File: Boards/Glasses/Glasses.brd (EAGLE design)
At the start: 157.5 x 68.6 mm, 260 parts, among them U1 APA1022020, U10 APA1022020, U100 APA1022020, U101 APA1022020, U102 APA1022020, U103 APA1022020, U104 APA1022020, U105 APA1022020, U106 APA1022020, U107 APA1022020, U108 APA1022020, U109 APA1022020, U11 APA1022020, U110 APA1022020, U111 APA1022020, U112 APA1022020, U113 APA1022020, U114 APA1022020, U115 APA1022020, U116 APA1022020, U117 APA1022020, U118 APA1022020, U119 APA1022020, U12 APA1022020, U120 APA1022020, U121 APA1022020, U122 APA1022020, U123 APA1022020, U124 APA1022020, U125 APA1022020, U126 APA1022020, U127 APA1022020, U128 APA1022020, U129 APA1022020, U13 APA1022020, U130 APA1022020, U131 APA1022020, U132 APA1022020, U133 APA1022020, U134 APA1022020, U135 APA1022020, U136 APA1022020, U137 APA1022020, U138 APA1022020, U139 APA1022020, U14 APA1022020, U140 APA1022020, U141 APA1022020, U142 APA1022020, U143 APA1022020, U144 APA1022020, U145 APA1022020, U146 APA1022020, U147 APA1022020, U148 APA1022020, U149 APA1022020, U15 APA1022020, U150 APA1022020, U151 APA1022020, U152 APA1022020, U153 APA1022020, U154 APA1022020, U155 APA1022020, U156 APA1022020, U157 APA1022020, U158 APA1022020, U159 APA1022020, U16 APA1022020, U160 APA1022020, U161 APA1022020, U162 APA1022020, U163 APA1022020, U164 APA1022020, U165 APA1022020, U166 APA1022020, U167 APA1022020, U168 APA1022020, U169 APA1022020, U17 APA1022020, U170 APA1022020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

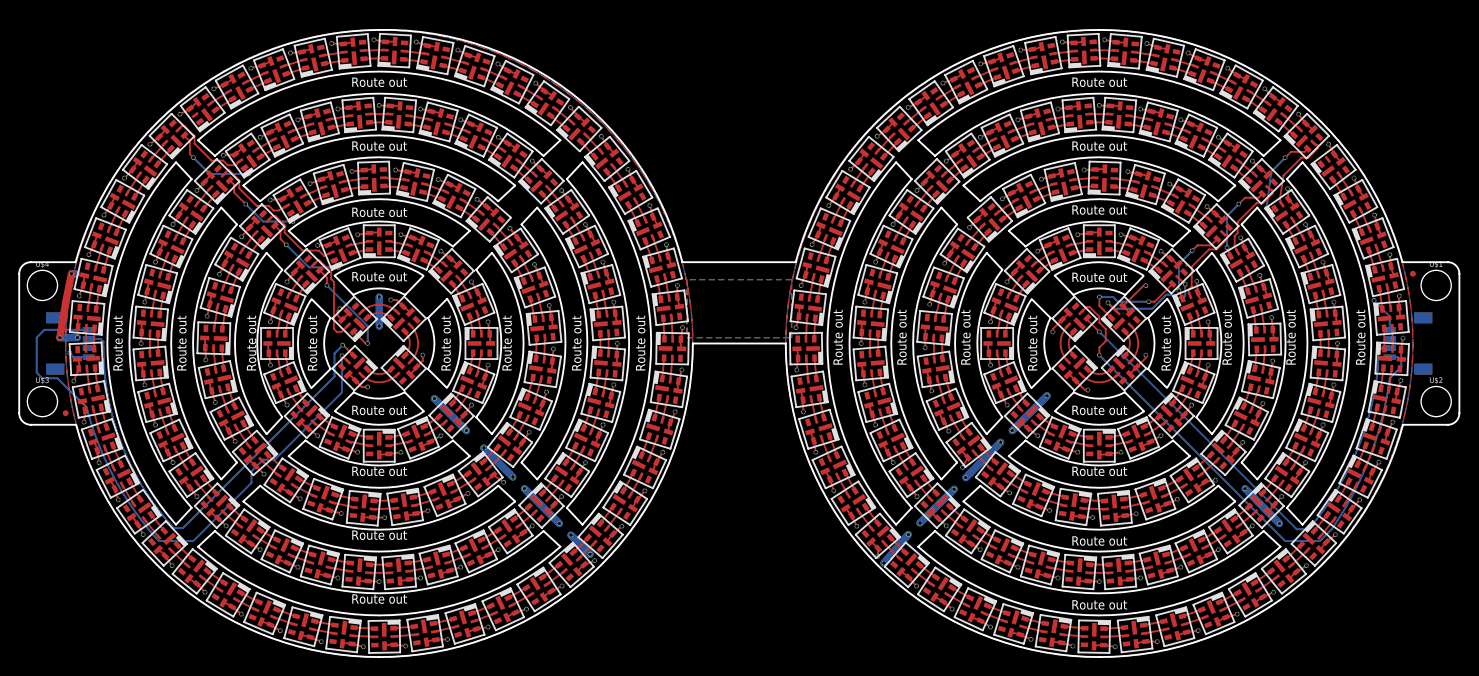
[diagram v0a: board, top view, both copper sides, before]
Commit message: adding gcode
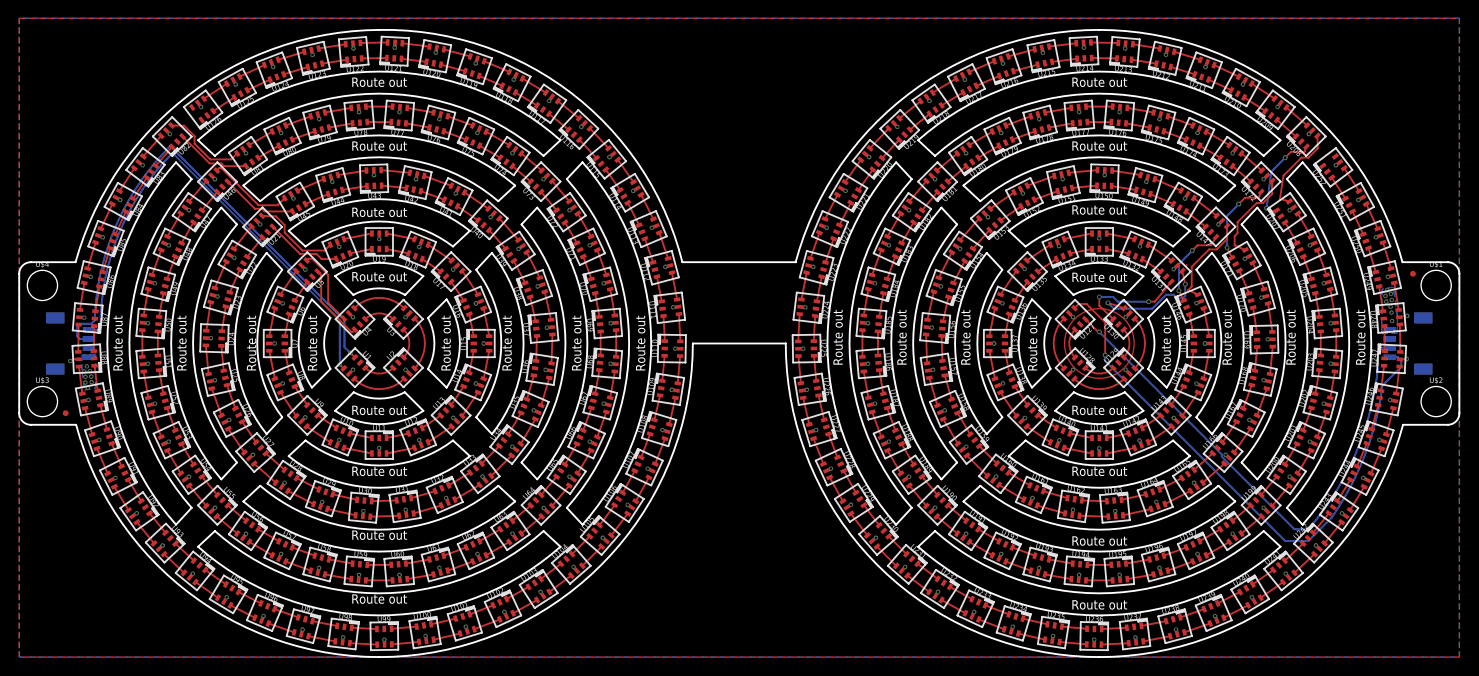
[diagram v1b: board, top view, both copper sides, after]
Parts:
- U1, U10, U100, U101, U102, U103, U104, U105, U106, U107, U108, U109, U11, U110, U111, U112, U113, U114, U115, U116, U117, U118, U119, U12, U120, U121, U122, U123, U124, U125, U126, U127, U128, U129, U13, U130, U131, U132, U133, U134, U135, U136, U137, U138, U139, U14, U140, U141, U142, U143, U144, U145, U146, U147, U148, U149, U15, U150, U151, U152, U153, U154, U155, U156, U157, U158, U159, U16, U160, U161, U162, U163, U164, U165, U166, U167, U168, U169, U17, U170, U171, U172, U173, U174, U175, U176, U177, U178, U179, U18, U180, U181, U182, U183, U184, U185, U186, U187, U188, U189, U19, U190, U191, U192, U193, U194, U195, U196, U197, U198, U199, U2, U20, U200, U201, U202, U203, U204, U205, U206, U207, U208, U209, U21, U210, U211, U212, U213, U214, U215, U216, U217, U218, U219, U22, U220, U221, U222, U223, U224, U225, U226, U227, U228, U229, U23, U230, U231, U232, U233, U234, U235, U236, U237, U238, U239, U24, U240, U241, U242, U243, U244, U245, U246, U247, U248, U249, U25, U250, U251, U252, U26, U27, U28, U29, U3, U30, U31, U32, U33, U34, U35, U36, U37, U38, U39, U4, U40, U41, U42, U43, U44, U45, U46, U47, U48, U49, U5, U50, U51, U52, U53, U54, U55, U56, U57, U58, U59, U6, U60, U61, U62, U63, U64, U65, U66, U67, U68, U69, U7, U70, U71, U72, U73, U74, U75, U76, U77, U78, U79, U8, U80, U81, U82, U83, U84, U85, U86, U87, U88, U89, U9, U90, U91, U92, U93, U94, U95, U96, U97, U98, U99: value APA1022020 -> APA102-2020; device 1_BES_Optoelectronics:APA102-2020 -> SparkFun-LED:APA102-2020
- turned U1 to 315 degrees
- turned U10 to 337.5 degrees
- turned U100 to 9 degrees
- turned U101 to 17 degrees
- turned U102 to 25 degrees
- turned U103 to 33 degrees
- turned U104 to 41 degrees
- turned U105 to 49 degrees
- turned U106 to 57 degrees
- turned U107 to 65 degrees
- turned U108 to 73 degrees
- turned U109 to 81 degrees
- turned U11 to 0 degrees
- turned U110 to 89 degrees
- turned U111 to 97 degrees
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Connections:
- net GND: no longer U1.GNDPAD, U10.GNDPAD, U100.GNDPAD, U101.GNDPAD, U102.GNDPAD, U103.GNDPAD, U104.GNDPAD, U105.GNDPAD, U106.GNDPAD, U107.GNDPAD, U108.GNDPAD, U109.GNDPAD, U11.GNDPAD, U110.GNDPAD, U111.GNDPAD, U112.GNDPAD, U113.GNDPAD, U114.GNDPAD, U115.GNDPAD, U116.GNDPAD, U117.GNDPAD, U118.GNDPAD, U119.GNDPAD, U12.GNDPAD, U120.GNDPAD, U121.GNDPAD, U122.GNDPAD, U123.GNDPAD, U124.GNDPAD, U125.GNDPAD, U126.GNDPAD, U127.GNDPAD, U128.GNDPAD, U129.GNDPAD, U13.GNDPAD, U130.GNDPAD, U131.GNDPAD, U132.GNDPAD, U133.GNDPAD, U134.GNDPAD, U135.GNDPAD, U136.GNDPAD, U137.GNDPAD, U138.GNDPAD, U139.GNDPAD, U14.GNDPAD, U140.GNDPAD, U141.GNDPAD, U142.GNDPAD, U143.GNDPAD, U144.GNDPAD, U145.GNDPAD, U146.GNDPAD, U147.GNDPAD, U148.GNDPAD, U149.GNDPAD, U15.GNDPAD, U150.GNDPAD, U151.GNDPAD, U152.GNDPAD, U153.GNDPAD, U154.GNDPAD, U155.GNDPAD, U156.GNDPAD, U157.GNDPAD, U158.GNDPAD, U159.GNDPAD, U16.GNDPAD, U160.GNDPAD, U161.GNDPAD, U162.GNDPAD, U163.GNDPAD, U164.GNDPAD, U165.GNDPAD, U166.GNDPAD, U167.GNDPAD, U168.GNDPAD, U169.GNDPAD, U17.GNDPAD, U170.GNDPAD, U171.GNDPAD, U172.GNDPAD, U173.GNDPAD, U174.GNDPAD, U175.GNDPAD, U176.GNDPAD, U177.GNDPAD, U178.GNDPAD, U179.GNDPAD, U18.GNDPAD, U180.GNDPAD, U181.GNDPAD, U182.GNDPAD, U183.GNDPAD, U184.GNDPAD, U185.GNDPAD, U186.GNDPAD, U187.GNDPAD, U188.GNDPAD, U189.GNDPAD, U19.GNDPAD, U190.GNDPAD, U191.GNDPAD, U192.GNDPAD, U193.GNDPAD, U194.GNDPAD, U195.GNDPAD, U196.GNDPAD, U197.GNDPAD, U198.GNDPAD, U199.GNDPAD, U2.GNDPAD, U20.GNDPAD, U200.GNDPAD, U201.GNDPAD, U202.GNDPAD, U203.GNDPAD, U204.GNDPAD, U205.GNDPAD, U206.GNDPAD, U207.GNDPAD, U208.GNDPAD, U209.GNDPAD, U21.GNDPAD, U210.GNDPAD, U211.GNDPAD, U212.GNDPAD, U213.GNDPAD, U214.GNDPAD, U215.GNDPAD, U216.GNDPAD, U217.GNDPAD, U218.GNDPAD, U219.GNDPAD, U22.GNDPAD, U220.GNDPAD, U221.GNDPAD, U222.GNDPAD, U223.GNDPAD, U224.GNDPAD, U225.GNDPAD, U226.GNDPAD, U227.GNDPAD, U228.GNDPAD, U229.GNDPAD, U23.GNDPAD, U230.GNDPAD, U231.GNDPAD, U232.GNDPAD, U233.GNDPAD, U234.GNDPAD, U235.GNDPAD, U236.GNDPAD, U237.GNDPAD, U238.GNDPAD, U239.GNDPAD, U24.GNDPAD, U240.GNDPAD, U241.GNDPAD, U242.GNDPAD, U243.GNDPAD, U244.GNDPAD, U245.GNDPAD, U246.GNDPAD, U247.GNDPAD, U248.GNDPAD, U249.GNDPAD, U25.GNDPAD, U250.GNDPAD, U251.GNDPAD, U252.GNDPAD, U26.GNDPAD, U27.GNDPAD, U28.GNDPAD, U29.GNDPAD, U3.GNDPAD, U30.GNDPAD, U31.GNDPAD, U32.GNDPAD, U33.GNDPAD, U34.GNDPAD, U35.GNDPAD, U36.GNDPAD, U37.GNDPAD, U38.GNDPAD, U39.GNDPAD, U4.GNDPAD, U40.GNDPAD, U41.GNDPAD, U42.GNDPAD, U43.GNDPAD, U44.GNDPAD, U45.GNDPAD, U46.GNDPAD, U47.GNDPAD, U48.GNDPAD, U49.GNDPAD, U5.GNDPAD, U50.GNDPAD, U51.GNDPAD, U52.GNDPAD, U53.GNDPAD, U54.GNDPAD, U55.GNDPAD, U56.GNDPAD, U57.GNDPAD, U58.GNDPAD, U59.GNDPAD, U6.GNDPAD, U60.GNDPAD, U61.GNDPAD, U62.GNDPAD, U63.GNDPAD, U64.GNDPAD, U65.GNDPAD, U66.GNDPAD, U67.GNDPAD, U68.GNDPAD, U69.GNDPAD, U7.GNDPAD, U70.GNDPAD, U71.GNDPAD, U72.GNDPAD, U73.GNDPAD, U74.GNDPAD, U75.GNDPAD, U76.GNDPAD, U77.GNDPAD, U78.GNDPAD, U79.GNDPAD, U8.GNDPAD, U80.GNDPAD, U81.GNDPAD, U82.GNDPAD, U83.GNDPAD, U84.GNDPAD, U85.GNDPAD, U86.GNDPAD, U87.GNDPAD, U88.GNDPAD, U89.GNDPAD, U9.GNDPAD, U90.GNDPAD, U91.GNDPAD, U92.GNDPAD, U93.GNDPAD, U94.GNDPAD, U95.GNDPAD, U96.GNDPAD, U97.GNDPAD, U98.GNDPAD, U99.GNDPAD
- net VCC: no longer U1.VDDPAD, U10.VDDPAD, U100.VDDPAD, U101.VDDPAD, U102.VDDPAD, U103.VDDPAD, U104.VDDPAD, U105.VDDPAD, U106.VDDPAD, U107.VDDPAD, U108.VDDPAD, U109.VDDPAD, U11.VDDPAD, U110.VDDPAD, U111.VDDPAD, U112.VDDPAD, U113.VDDPAD, U114.VDDPAD, U115.VDDPAD, U116.VDDPAD, U117.VDDPAD, U118.VDDPAD, U119.VDDPAD, U12.VDDPAD, U120.VDDPAD, U121.VDDPAD, U122.VDDPAD, U123.VDDPAD, U124.VDDPAD, U125.VDDPAD, U126.VDDPAD, U127.VDDPAD, U128.VDDPAD, U129.VDDPAD, U13.VDDPAD, U130.VDDPAD, U131.VDDPAD, U132.VDDPAD, U133.VDDPAD, U134.VDDPAD, U135.VDDPAD, U136.VDDPAD, U137.VDDPAD, U138.VDDPAD, U139.VDDPAD, U14.VDDPAD, U140.VDDPAD, U141.VDDPAD, U142.VDDPAD, U143.VDDPAD, U144.VDDPAD, U145.VDDPAD, U146.VDDPAD, U147.VDDPAD, U148.VDDPAD, U149.VDDPAD, U15.VDDPAD, U150.VDDPAD, U151.VDDPAD, U152.VDDPAD, U153.VDDPAD, U154.VDDPAD, U155.VDDPAD, U156.VDDPAD, U157.VDDPAD, U158.VDDPAD, U159.VDDPAD, U16.VDDPAD, U160.VDDPAD, U161.VDDPAD, U162.VDDPAD, U163.VDDPAD, U164.VDDPAD, U165.VDDPAD, U166.VDDPAD, U167.VDDPAD, U168.VDDPAD, U169.VDDPAD, U17.VDDPAD, U170.VDDPAD, U171.VDDPAD, U172.VDDPAD, U173.VDDPAD, U174.VDDPAD, U175.VDDPAD, U176.VDDPAD, U177.VDDPAD, U178.VDDPAD, U179.VDDPAD, U18.VDDPAD, U180.VDDPAD, U181.VDDPAD, U182.VDDPAD, U183.VDDPAD, U184.VDDPAD, U185.VDDPAD, U186.VDDPAD, U187.VDDPAD, U188.VDDPAD, U189.VDDPAD, U19.VDDPAD, U190.VDDPAD, U191.VDDPAD, U192.VDDPAD, U193.VDDPAD, U194.VDDPAD, U195.VDDPAD, U196.VDDPAD, U197.VDDPAD, U198.VDDPAD, U199.VDDPAD, U2.VDDPAD, U20.VDDPAD, U200.VDDPAD, U201.VDDPAD, U202.VDDPAD, U203.VDDPAD, U204.VDDPAD, U205.VDDPAD, U206.VDDPAD, U207.VDDPAD, U208.VDDPAD, U209.VDDPAD, U21.VDDPAD, U210.VDDPAD, U211.VDDPAD, U212.VDDPAD, U213.VDDPAD, U214.VDDPAD, U215.VDDPAD, U216.VDDPAD, U217.VDDPAD, U218.VDDPAD, U219.VDDPAD, U22.VDDPAD, U220.VDDPAD, U221.VDDPAD, U222.VDDPAD, U223.VDDPAD, U224.VDDPAD, U225.VDDPAD, U226.VDDPAD, U227.VDDPAD, U228.VDDPAD, U229.VDDPAD, U23.VDDPAD, U230.VDDPAD, U231.VDDPAD, U232.VDDPAD, U233.VDDPAD, U234.VDDPAD, U235.VDDPAD, U236.VDDPAD, U237.VDDPAD, U238.VDDPAD, U239.VDDPAD, U24.VDDPAD, U240.VDDPAD, U241.VDDPAD, U242.VDDPAD, U243.VDDPAD, U244.VDDPAD, U245.VDDPAD, U246.VDDPAD, U247.VDDPAD, U248.VDDPAD, U249.VDDPAD, U25.VDDPAD, U250.VDDPAD, U251.VDDPAD, U252.VDDPAD, U26.VDDPAD, U27.VDDPAD, U28.VDDPAD, U29.VDDPAD, U3.VDDPAD, U30.VDDPAD, U31.VDDPAD, U32.VDDPAD, U33.VDDPAD, U34.VDDPAD, U35.VDDPAD, U36.VDDPAD, U37.VDDPAD, U38.VDDPAD, U39.VDDPAD, U4.VDDPAD, U40.VDDPAD, U41.VDDPAD, U42.VDDPAD, U43.VDDPAD, U44.VDDPAD, U45.VDDPAD, U46.VDDPAD, U47.VDDPAD, U48.VDDPAD, U49.VDDPAD, U5.VDDPAD, U50.VDDPAD, U51.VDDPAD, U52.VDDPAD, U53.VDDPAD, U54.VDDPAD, U55.VDDPAD, U56.VDDPAD, U57.VDDPAD, U58.VDDPAD, U59.VDDPAD, U6.VDDPAD, U60.VDDPAD, U61.VDDPAD, U62.VDDPAD, U63.VDDPAD, U64.VDDPAD, U65.VDDPAD, U66.VDDPAD, U67.VDDPAD, U68.VDDPAD, U69.VDDPAD, U7.VDDPAD, U70.VDDPAD, U71.VDDPAD, U72.VDDPAD, U73.VDDPAD, U74.VDDPAD, U75.VDDPAD, U76.VDDPAD, U77.VDDPAD, U78.VDDPAD, U79.VDDPAD, U8.VDDPAD, U80.VDDPAD, U81.VDDPAD, U82.VDDPAD, U83.VDDPAD, U84.VDDPAD, U85.VDDPAD, U86.VDDPAD, U87.VDDPAD, U88.VDDPAD, U89.VDDPAD, U9.VDDPAD, U90.VDDPAD, U91.VDDPAD, U92.VDDPAD, U93.VDDPAD, U94.VDDPAD, U95.VDDPAD, U96.VDDPAD, U97.VDDPAD, U98.VDDPAD, U99.VDDPAD
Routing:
- net VCC: track 600.4 -> 136.7 mm, vias 254 -> 252
- net GND: track 52.8 -> 0.06 mm, vias 22 -> 16
- net N$490: track 65.9 -> 53.3 mm
- net N$8: track 12.3 -> 8.62 mm, vias 2 -> 0
- net N$270: track 53.5 -> 56.9 mm
- net N$7: track 10.9 -> 8.65 mm
- net N$154: track 10.4 -> 8.30 mm, vias 2 -> 0
- net N$38: track 10.2 -> 8.40 mm, vias 2 -> 0
- net N$85: track 10.2 -> 8.45 mm, vias 2 -> 0
- net N$245: track 3.90 -> 5.46 mm
- net N$6: track 3.90 -> 5.46 mm
- net N$3: track 3.90 -> 5.46 mm
- net N$248: track 3.90 -> 5.46 mm
- net N$244: track 3.90 -> 5.46 mm
- net N$2: track 3.90 -> 5.46 mm
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- added copper zone on layer 16, net GND
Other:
- outline, holes or cut-outs redrawn
